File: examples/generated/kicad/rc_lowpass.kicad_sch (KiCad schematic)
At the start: 3 parts

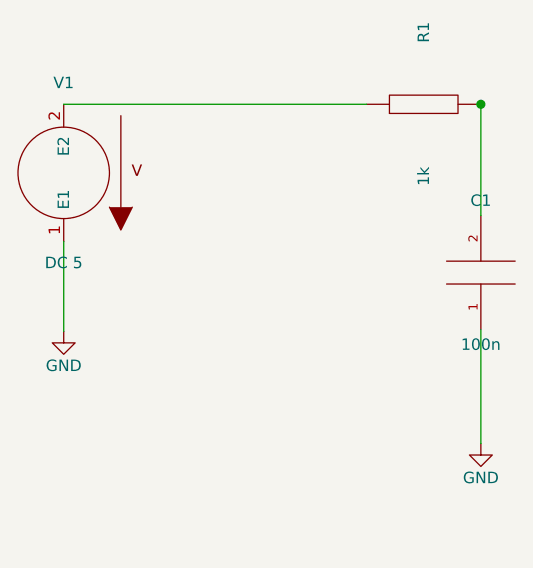
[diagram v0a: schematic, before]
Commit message: Attempt to fix more terminal issues.
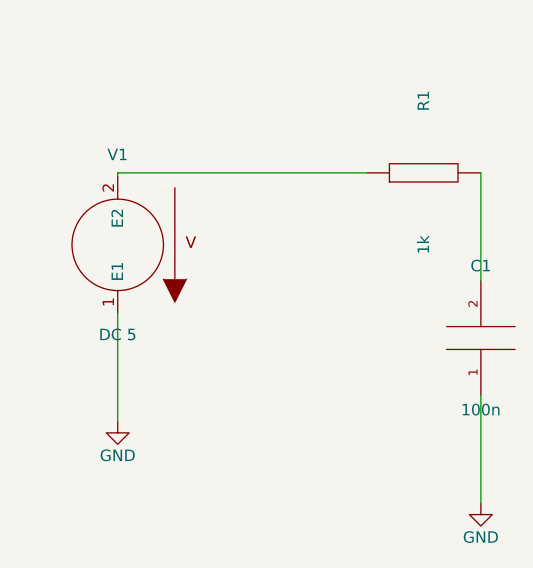
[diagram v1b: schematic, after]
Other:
- moved on the sheet: C1, R1, V1
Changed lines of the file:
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@@
     (comment 1 "Generated by mixedsig2cad")
   )
-  (symbol (lib_id "VSOURCE") (at 50.00 78.00 180) (unit 1)
+  (symbol (lib_id "VSOURCE") (at 56.00 86.00 180) (unit 1)
     (in_bom yes) (on_board yes)
-    (property "Reference" "V1" (at 50.0 68.0 0)
+    (property "Reference" "V1" (at 56.0 76.0 0)
       (effects (font (size 1.27 1.27)))
     )
-    (property "Value" "DC 5" (at 50.0 88.0 0)
+    (property "Value" "DC 5" (at 56.0 96.0 0)
       (effects (font (size 1.27 1.27)))
     )
@@
     )
   )
-  (symbol (lib_id "R") (at 90.00 70.38 90) (unit 1)
+  (symbol (lib_id "GND") (at 56.00 105.62 0) (unit 1)
     (in_bom yes) (on_board yes)
-    (property "Reference" "R1" (at 90.0 62.379999999999995 0)
-      (effects (font (size 1.27 1.27)))
+    (property "Reference" "#PWR0001" (at 56.0 101.81 0)
+      (effects (font (size 1.27 1.27)) hide)
     )
-    (property "Value" "1k" (at 90.0 78.38 0)
+    (property "Value" "GND" (at 56.0 109.43 0)
       (effects (font (size 1.27 1.27)))
     )
@@
     )
   )
-  (symbol (lib_id "CAP") (at 96.35 89.08 180) (unit 1)
+  (symbol (lib_id "R") (at 90.00 78.00 90) (unit 1)
     (in_bom yes) (on_board yes)
-    (property "Reference" "C1" (at 96.35 81.08 0)
+    (property "Reference" "R1" (at 90.0 70.0 0)
       (effects (font (size 1.27 1.27)))
     )
-    (property "Value" "100n" (at 96.35 97.08 0)
+    (property "Value" "1k" (at 90.0 86.0 0)
       (effects (font (size 1.27 1.27)))
     )
@@
     )
   )
-  (symbol (lib_id "GND") (at 50.00 95.62 0) (unit 1)
+  (symbol (lib_id "CAP") (at 96.35 96.35 180) (unit 1)
     (in_bom yes) (on_board yes)
-    (property "Reference" "#PWR0001" (at 50.0 91.81 0)
-      (effects (font (size 1.27 1.27)) hide)
+    (property "Reference" "C1" (at 96.35 88.35 0)
+      (effects (font (size 1.27 1.27)))
     )
-    (property "Value" "GND" (at 50.0 99.43 0)
+    (property "Value" "100n" (at 96.35 104.35 0)
       (effects (font (size 1.27 1.27)))
     )
@@
     )
   )
-  (symbol (lib_id "GND") (at 96.35 108.08 0) (unit 1)
+  (symbol (lib_id "GND") (at 96.35 114.70 0) (unit 1)
     (in_bom yes) (on_board yes)
-    (property "Reference" "#PWR0002" (at 96.35 104.27 0)
+    (property "Reference" "#PWR0002" (at 96.35 110.89 0)
       (effects (font (size 1.27 1.27)) hide)
     )
-    (property "Value" "GND" (at 96.35 111.89 0)
+    (property "Value" "GND" (at 96.35 118.51 0)
       (effects (font (size 1.27 1.27)))
     )
@@
     )
   )
-  (wire (pts (xy 50.00 70.38) (xy 83.65 70.38))
+  (wire (pts (xy 96.35 102.70) (xy 96.35 114.70))
     (stroke (width 0) (type solid) (color 0 0 0 0))
   )
-  (wire (pts (xy 96.35 82.73) (xy 96.35 70.38))
+  (wire (pts (xy 56.00 93.62) (xy 56.00 105.62))
     (stroke (width 0) (type solid) (color 0 0 0 0))
   )
-  (wire (pts (xy 50.00 85.62) (xy 50.00 95.62))
+  (wire (pts (xy 56.00 78.38) (xy 56.00 78.00))
     (stroke (width 0) (type solid) (color 0 0 0 0))
   )
-  (wire (pts (xy 96.35 95.43) (xy 96.35 108.08))
+  (wire (pts (xy 56.00 78.00) (xy 83.65 78.00))
     (stroke (width 0) (type solid) (color 0 0 0 0))
   )
-  (junction (at 96.35 70.38) (diameter 1.016) (color 0 0 0 0))
+  (wire (pts (xy 96.35 78.00) (xy 96.35 90.00))
+    (stroke (width 0) (type solid) (color 0 0 0 0))
+  )
   (sheet_instances
     (path "/" (page "1"))
@@
   (symbol_instances
     (path "/c171cc21-d2ba-581e-8446-b23465a59c7b" (reference "V1") (unit 1) (value "DC 5") (footprint ""))
+    (path "/99395be3-a0e4-5d09-bc7f-547778482ecc" (reference "#PWR0001") (unit 1) (value "GND") (footprint ""))
     (path "/f9364b86-dfb1-51e8-9247-72a2484cf109" (reference "R1") (unit 1) (value "1k") (footprint ""))
     (path "/fff04eb7-92e3-5e3e-9950-c8b8ac3c6096" (reference "C1") (unit 1) (value "100n") (footprint ""))
-    (path "/99395be3-a0e4-5d09-bc7f-547778482ecc" (reference "#PWR0001") (unit 1) (value "GND") (footprint ""))
     (path "/662a2282-d2d1-5b8b-9fa8-19311be8b5b1" (reference "#PWR0002") (unit 1) (value "GND") (footprint ""))
   )
